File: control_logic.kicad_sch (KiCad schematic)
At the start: 71 parts, among them J12 SWD Header, J17 TC2050, SW1 TS342A2P, SW2 TS342A2P, U1 INA181A1, U10 L7805, U11 MCP2562-E-SN, U12 STM32F105RCTx, U13 AZ1117I-3.3, U15 TPD4E1U06, Y3 8MHz 12pF

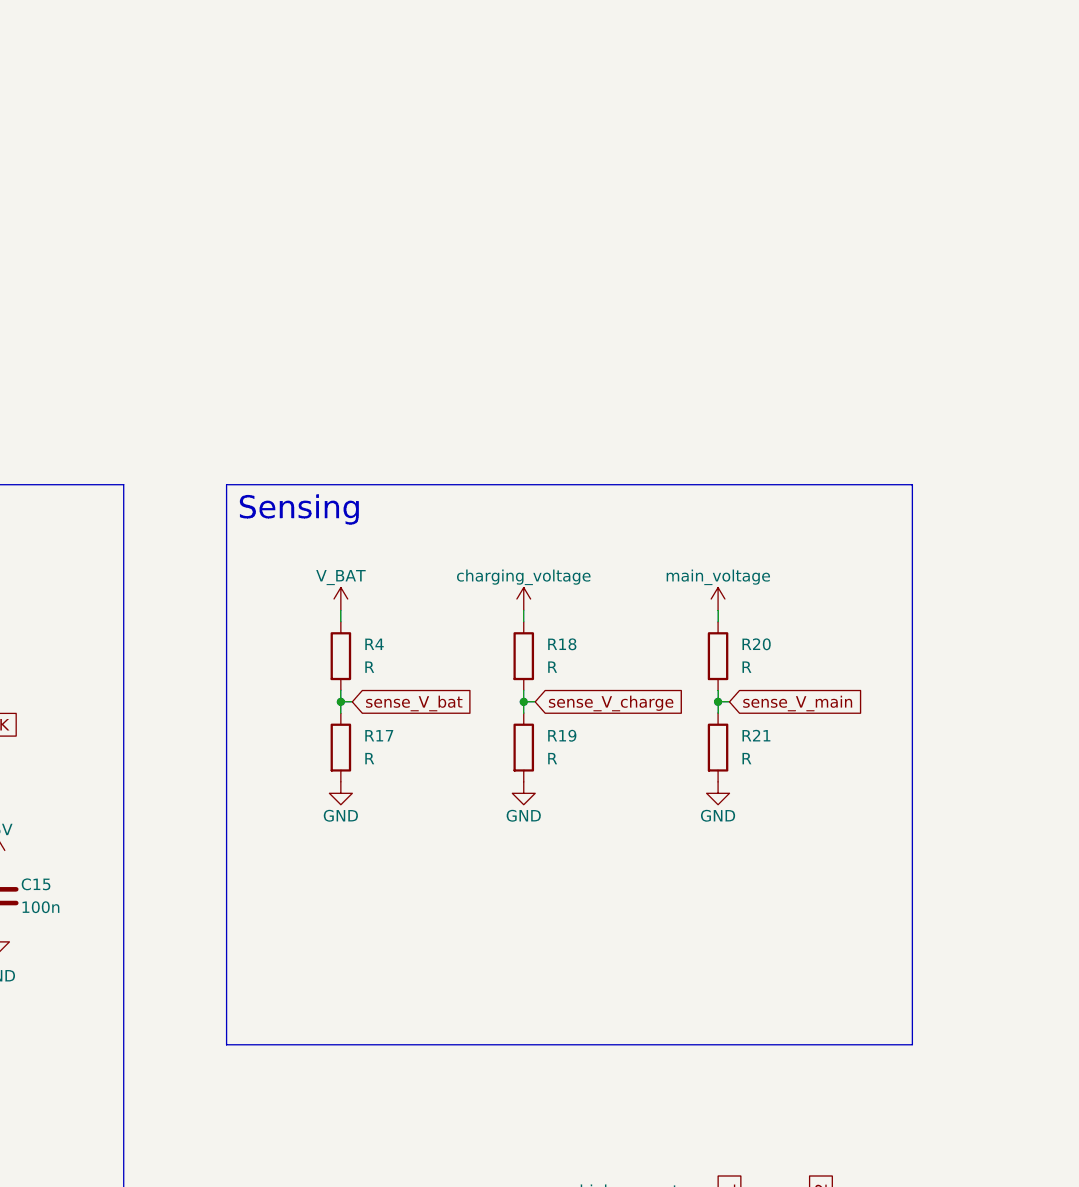
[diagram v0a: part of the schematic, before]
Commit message: calculated sensing-resistor values
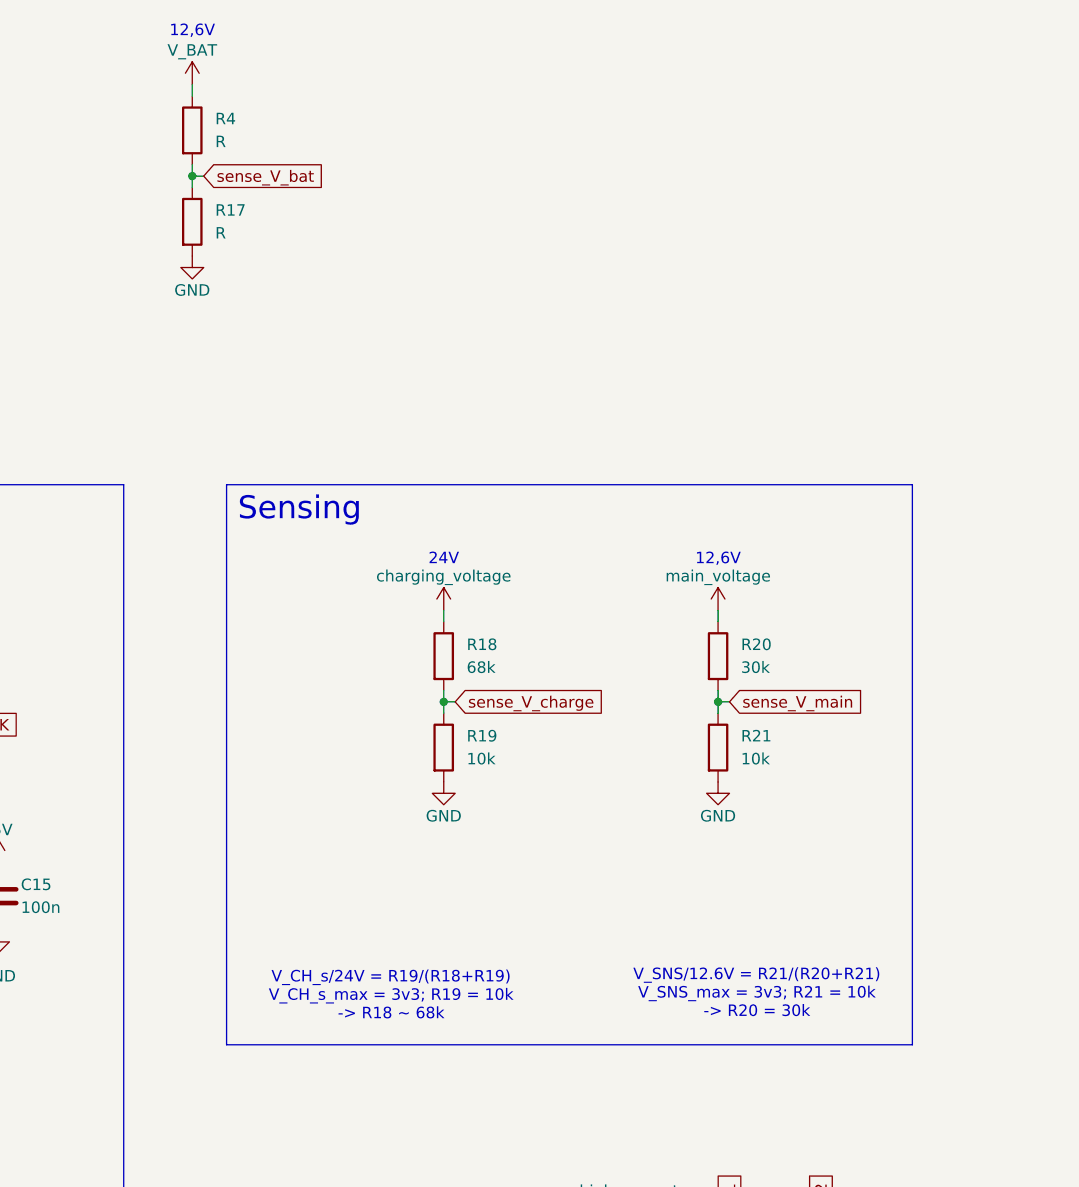
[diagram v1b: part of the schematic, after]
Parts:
- R18: value R -> 68k; footprint (none) -> Resistor_SMD:R_0603_1608Metric; LCSC (none) -> C23231
- R19, R21: value R -> 10k; footprint (none) -> Resistor_SMD:R_0402_1005Metric; LCSC (none) -> C25744
- R20: value R -> 30k; footprint (none) -> Resistor_SMD:R_0603_1608Metric; LCSC (none) -> C22984
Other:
- note added: "12,6V"
- note added: "24V"
- note added: "V_CH_s/24V = R19/(R18+R19) V_CH_s_max = 3v3; R19 = 10k -> R18 ~ 68k"
- note added: "V_SNS/12.6V = R21/(R20+R21) V_SNS_max = 3v3; R21 = 10k -> R20 = 30k"
- moved on the sheet: R17, R18, R19, R4
